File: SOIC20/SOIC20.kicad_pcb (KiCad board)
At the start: 2 copper layers, 25.7 x 18 mm, 7 parts, among them J1 Conn_01x10, J2 Conn_02x10_Counter_Clockwise, J4 Conn_02x10_Counter_Clockwise, J5 Conn_01x10

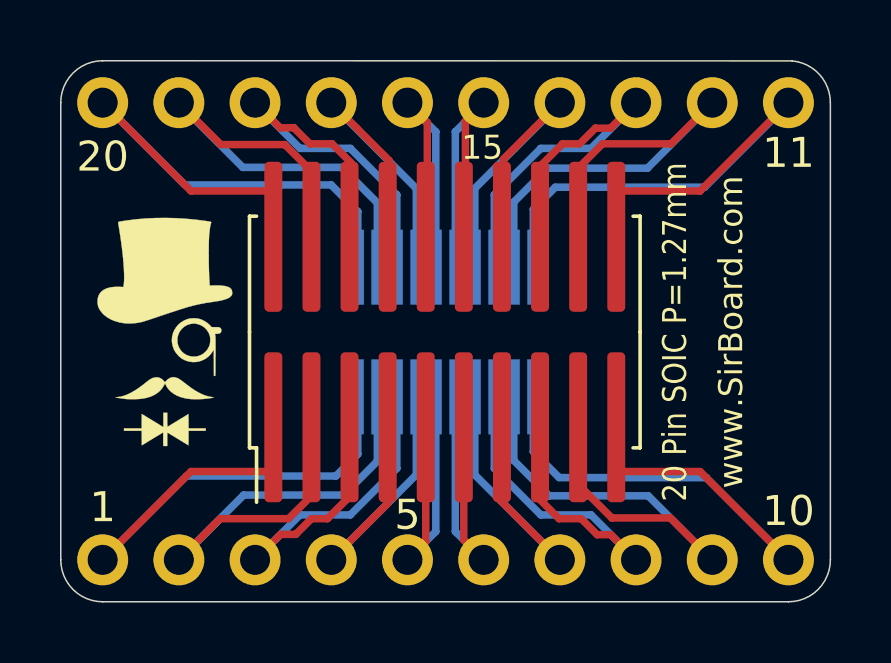
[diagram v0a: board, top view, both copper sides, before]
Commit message: Board Updates
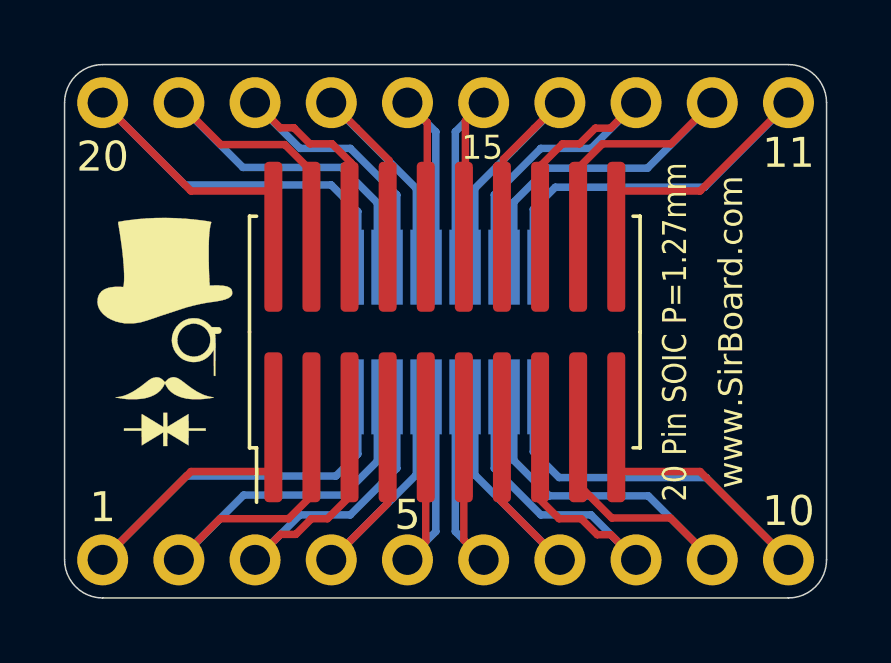
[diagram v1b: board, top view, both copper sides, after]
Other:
- board size 25.7 x 18 mm -> 25.4 x 17.8 mm
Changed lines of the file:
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@@
       (xy -0.06096 3.169456) (xy -0.06096 2.6924) (xy 0.07112 2.6924) (xy 0.07112 2.926926)) (layer F.SilkS) (width 0.01))
   )
+  (gr_line (start 77.089 43.7896) (end 77.089 28.5496) (layer Edge.Cuts) (width 0.05))
+  (gr_line (start 52.959 45.0596) (end 75.819 45.0596) (layer Edge.Cuts) (width 0.05))
+  (gr_line (start 51.689 28.5496) (end 51.689 43.7896) (layer Edge.Cuts) (width 0.05))
+  (gr_line (start 75.819 27.2796) (end 52.959 27.2796) (layer Edge.Cuts) (width 0.05))
+  (gr_arc (start 75.819 28.5496) (end 77.089 28.5496) (angle -90) (layer Edge.Cuts) (width 0.05))
+  (gr_arc (start 75.819 43.7896) (end 75.819 45.0596) (angle -90) (layer Edge.Cuts) (width 0.05))
+  (gr_arc (start 52.959 43.7896) (end 51.689 43.7896) (angle -90) (layer Edge.Cuts) (width 0.05))
+  (gr_arc (start 52.959 28.5496) (end 52.959 27.2796) (angle -90) (layer Edge.Cuts) (width 0.05))
   (dimension 18.034 (width 0.15) (layer Dwgs.User)
     (gr_text "18.034 mm" (at 83.215 36.1696 90) (layer Dwgs.User)
@@
     (effects (font (size 0.8 0.7) (thickness 0.13)))
   )
-  (gr_line (start 77.216 43.7896) (end 77.216 28.5496) (layer Edge.Cuts) (width 0.05))
-  (gr_line (start 52.959 45.1866) (end 75.819 45.1866) (layer Edge.Cuts) (width 0.05))
-  (gr_line (start 51.562 28.5496) (end 51.562 43.7896) (layer Edge.Cuts) (width 0.05))
-  (gr_line (start 75.945478 27.158337) (end 52.959 27.1526) (layer Edge.Cuts) (width 0.05))
-  (gr_arc (start 75.819 28.5496) (end 77.216 28.5496) (angle -84.80557109) (layer Edge.Cuts) (width 0.05))
-  (gr_arc (start 75.819 43.7896) (end 75.819 45.1866) (angle -90) (layer Edge.Cuts) (width 0.05))
-  (gr_arc (start 52.959 43.7896) (end 51.562 43.7896) (angle -90) (layer Edge.Cuts) (width 0.05))
-  (gr_arc (start 52.959 28.5496) (end 52.959 27.1526) (angle -90) (layer Edge.Cuts) (width 0.05))
   (segment (start 72.8744 40.845) (end 75.819 43.7896) (width 0.25) (layer F.Cu) (net 1))
   (segment (start 70.0786 40.845) (end 72.8744 40.845) (width 0.25) (layer F.Cu) (net 1))
